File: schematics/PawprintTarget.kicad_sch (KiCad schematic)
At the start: 60 parts, among them J1 Conn_01x15, J2 Conn_01x15, J4 RJ45, J5 RJ45, J8 Motor, J9 Motor, Q1 2N7002BK, Q2 2N7002BK, SW1 SW_DIP_x04, SW2 SW_DIP_x04, U1 MAX485E, U2 EAIRMCA1, U3 Mini360

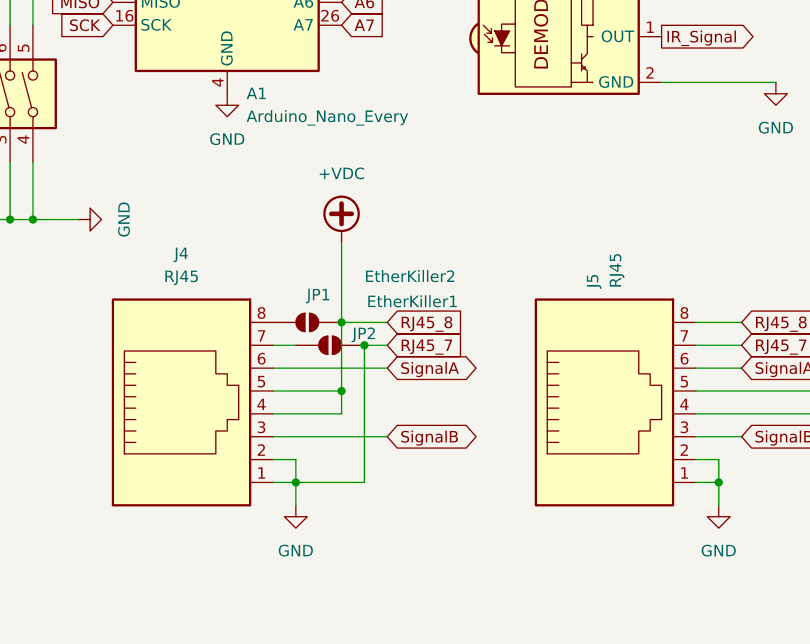
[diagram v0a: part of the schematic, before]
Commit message: Fix RJ45 connector
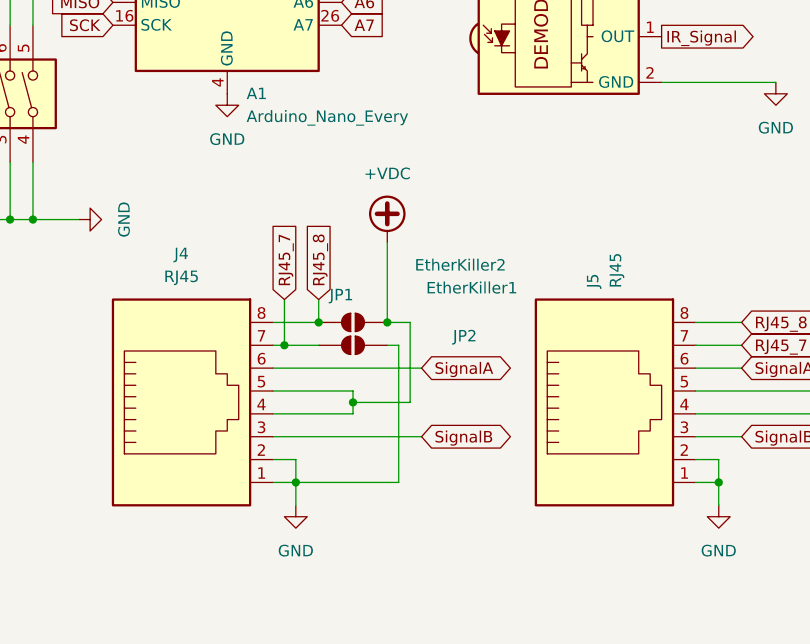
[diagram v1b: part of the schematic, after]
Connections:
- net +VDC: no longer J5.8
- net GND: no longer J5.7
- net RJ45_7: now reaches J4.7, JP1.1 (A)
- net RJ45_7: now also J5.7
- net RJ45_8: now reaches J4.8, JP2.1 (A)
- net RJ45_8: now also J5.8
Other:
- moved on the sheet: JP1, JP2

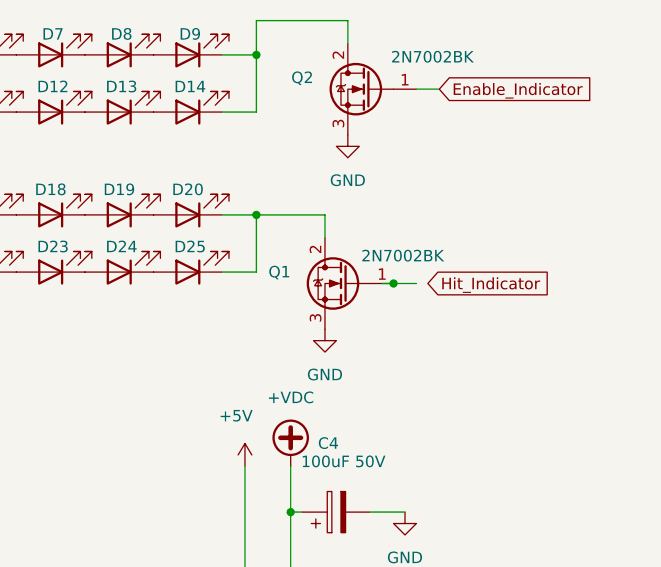
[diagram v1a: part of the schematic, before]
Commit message: Done, probably
- Nicer labels
- Probably won't blow up
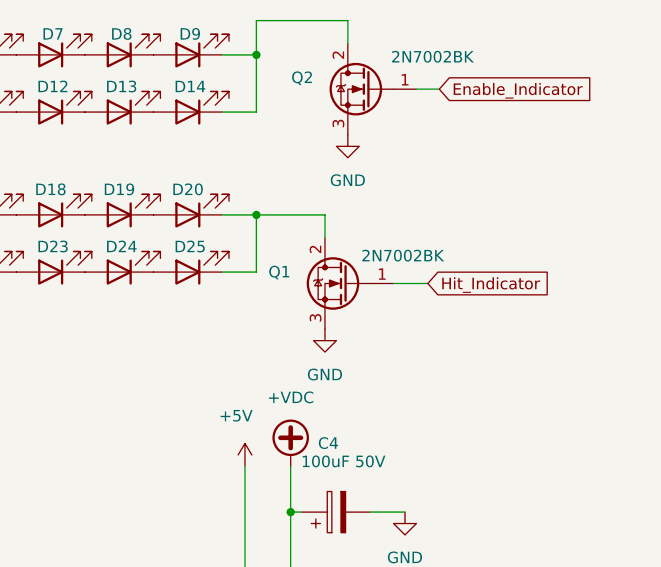
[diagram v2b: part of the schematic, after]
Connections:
- net Hit_Indicator: now also Q1.1 (G)
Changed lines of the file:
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@@
-	)
-	(junction
-		(at 264.16 85.09)
-		(diameter 0)
-		(color 0 0 0 0)
 	)
 	(junction
@@
 	(wire
 		(pts
-			(xy 264.16 85.09) (xy 262.89 85.09)
-		)
-		(stroke
-			(width 0)
-			(type default)
-		)
-	)
-	(wire
-		(pts
 			(xy 54.61 153.67) (xy 58.42 153.67)
 		)
@@
 	(wire
 		(pts
+			(xy 264.16 85.09) (xy 267.97 85.09)
+		)
+		(stroke
+			(width 0)
+			(type default)
+		)
+	)
+	(wire
+		(pts
 			(xy 58.42 115.57) (xy 54.61 115.57)
 		)
@@
 		)
 		(stroke
-			(width 0)
-			(type default)
-		)
-	)
-	(wire
-		(pts
-			(xy 266.7 85.09) (xy 264.16 85.09)
-		)
-		(stroke
